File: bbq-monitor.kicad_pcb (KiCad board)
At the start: 4 copper layers, 48.5 x 43.3 mm, 51 parts, among them J1 Power, J2 USB_B_Mini, J3 Thermocouple, Q1 AO3401A, Q2 BC847, Q3 BC847, SW1 SW_Push, U1 ESP32-WROOM-32D, U2 TPS62132, U3 CP2104, U4 USBLC6-2SC6, U5 AD8495, U6 DHT11

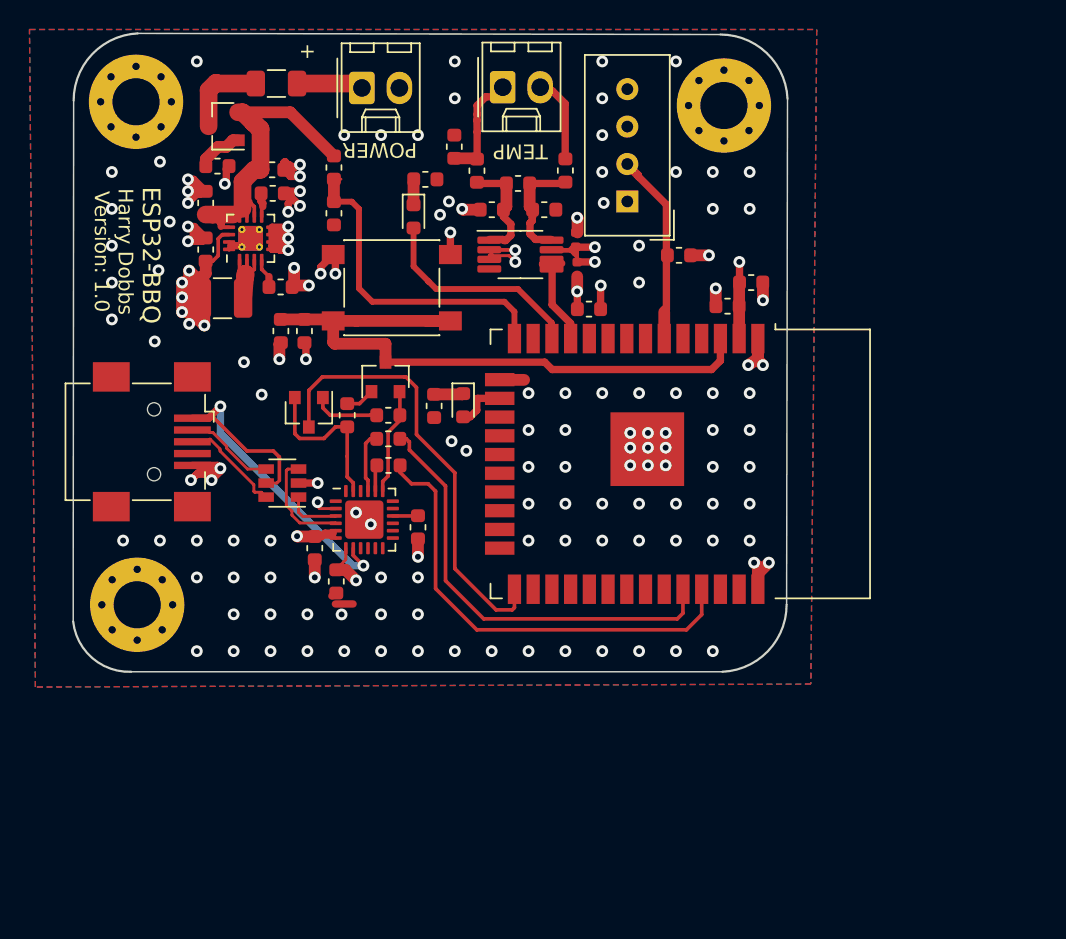
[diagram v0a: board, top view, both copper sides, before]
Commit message: up
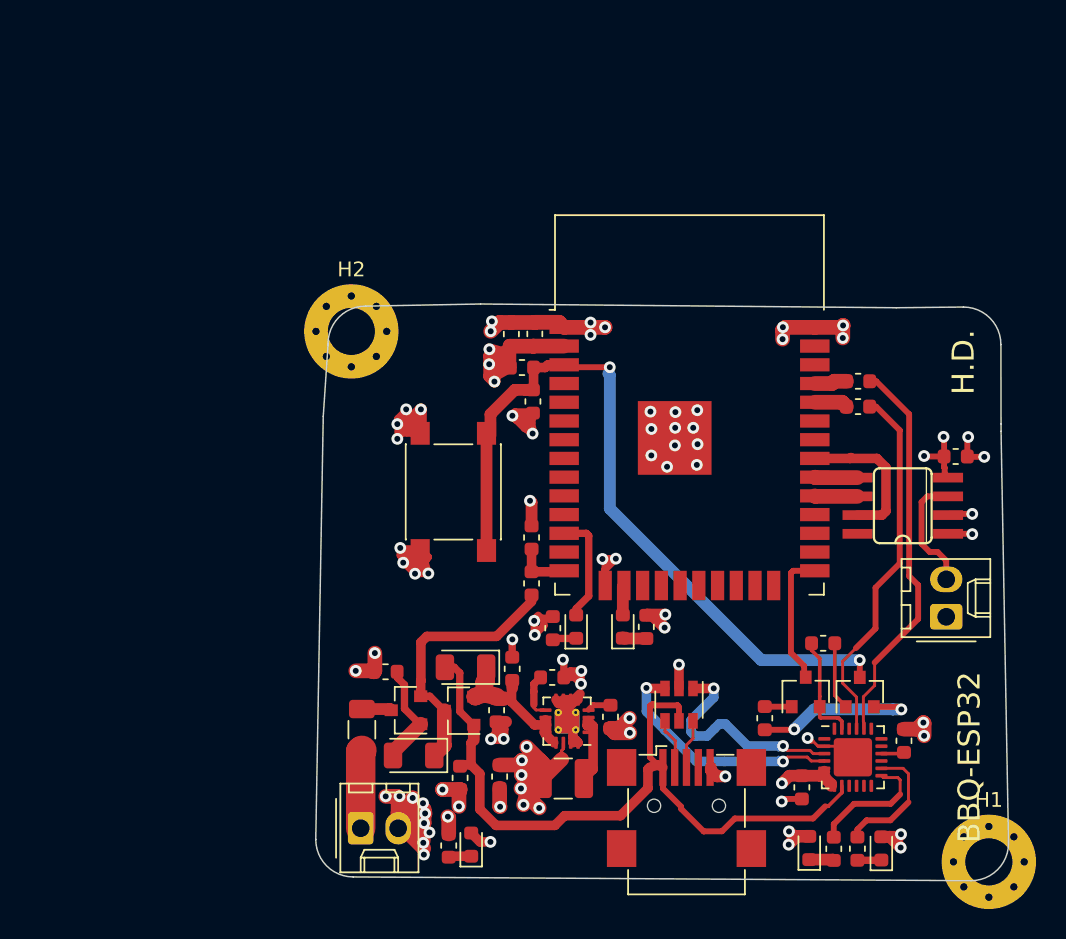
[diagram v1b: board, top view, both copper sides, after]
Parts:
- removed C10, C12, C14: 100n, Capacitor_SMD:C_0603_1608Metric
- removed C13, C15: 10n, Capacitor_SMD:C_0603_1608Metric
- removed C16: 100n, Capacitor_SMD:C_0402_1005Metric
- removed C17: 10u, Capacitor_SMD:C_0402_1005Metric
- removed H4: TR, MountingHole:MountingHole_3.2mm_M3_Pad_Via
- removed U5: AD8495, Package_SO:MSOP-8_3x3mm_P0.65mm
- removed U6: DHT11, Sensor:Aosong_DHT11_5.5x12.0_P2.54mm
- added C9: 100n, Capacitor_SMD:C_0603_1608Metric, F.Cu at (206.5, 86.8)
- added D3: RED, LED_SMD:LED_0603_1608Metric, F.Cu at (173.6, 113.1)
- added D4: RED, LED_SMD:LED_0603_1608Metric, F.Cu at (201.4, 113.4)
- added D5: RED, LED_SMD:LED_0603_1608Metric, F.Cu at (196.5, 113.4)
- added D6: D_Zener, Diode_SMD:D_1206_3216Metric, F.Cu at (169.7, 107.1)
- added D7: D_Schottky, Diode_SMD:D_1206_3216Metric, F.Cu at (173.2, 101.1)
- added IC1: MAX6675, hardware libraries:SO08, F.Cu at (202.9, 90.1)
- added Q4: AO3401A, Package_TO_SOT_SMD:SOT-23, F.Cu at (172.8, 104.0)
- J1: value Power -> Battery Power
- R10, R11, R9: value 1M -> 220
- R13: value 100 -> 10k
- moved H1 60.3 mm to (208.7, 114.3)
- moved R11 52.0 mm to (198.2, 113.4)
- moved J1 50.2 mm to (166.1, 112.0)
- moved R10 50.1 mm to (199.8, 113.4)
- moved R9 47.4 mm to (172.1, 113.2)
- moved J3 46.9 mm to (205.8, 97.7), turned to 90 degrees
- moved F1 44.2 mm to (166.2, 105.3), turned to 270 degrees
- moved J2 43.7 mm to (188.2, 110.5), turned to 0 degrees
- moved Q1 41.5 mm to (169.2, 104.0)
- moved C8 40.9 mm to (175.5, 108.5), turned to 270 degrees
- moved L1 39.9 mm to (179.9, 108.6)
- moved C1 39.7 mm to (175.3, 104.0), turned to 270 degrees
- moved U2 39.2 mm to (180.1, 104.8), turned to 180 degrees
- moved Q2 38.7 mm to (196.3, 102.8), turned to 90 degrees
- moved Q3 38.6 mm to (200.0, 102.8)
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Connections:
- net Net-(F1-Pad2) renamed BATT_PWR
- C1 pad 1: /BATT -> Net-(C1-Pad1)
- C2 pad 1: /BATT -> Net-(C1-Pad1)
- J2 pad 1: +5V -> USB_PWR
- J3 pad 1: Net-(J3-Pad1) -> GND
- J3 pad 2: Net-(J3-Pad2) -> Net-(IC1-Pad3)
- Q1 pad 2: /BATT -> BATT_SAFE
- R10 pad 1: Net-(J3-Pad2) -> TX_LED
- R10 pad 2: /Thermocouple_INPUT_FILTERED+ -> Net-(D4-Pad1)
- R11 pad 1: Net-(J3-Pad1) -> RX_LED
- R11 pad 2: /Thermocouple_INPUT_FILTERED- -> Net-(D5-Pad1)
- R12 pad 1: +3V3 -> GND
- R12 pad 2: TEMP_HUMID_SEN -> USB_PWR
- R14 pad 1: /BATT -> BATT_SAFE
- R9 pad 2: Net-(J3-Pad1) -> Net-(D3-Pad1)
- U1 pad 11: THERMOCOUPLE -> Net-(U1-Pad11)
- U1 pad 29: Net-(U1-Pad29) -> THERMO_SPI_CS
- U1 pad 30: Net-(U1-Pad30) -> THERMO_SPI_CLK
- U1 pad 31: Net-(U1-Pad31) -> THERMO_SPI_DO
- U1 pad 6: TEMP_HUMID_SEN -> Net-(U1-Pad6)
- U2 pad 10: /BATT -> Net-(C1-Pad1)
- U2 pad 11: /BATT -> Net-(C1-Pad1)
- U2 pad 12: /BATT -> Net-(C1-Pad1)
- U2 pad 13: /BATT -> Net-(C1-Pad1)
- U3 pad 13: Net-(U3-Pad13) -> RX_LED
- U3 pad 14: Net-(U3-Pad14) -> TX_LED
- U3 pad 8: +5V -> USB_PWR
- U4 pad 5: +5V -> USB_PWR
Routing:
- net USB_PWR: track 0.00 -> 51.1 mm
- net GND: track 71.2 -> 117.4 mm, vias 141 -> 68
- net /DIFF+: track 31.9 -> 2.22 mm
- net /DIFF-: track 30.7 -> 2.27 mm
- net +5V: track 27.4 -> 0.00 mm, vias 2 -> 0
- net /BATT: track 26.2 -> 0.00 mm
- net RX_CP+: track 1.78 -> 26.7 mm
- net GPIO0: track 30.3 -> 9.16 mm
- net TX_CP-: track 4.18 -> 24.9 mm
- net BATT_LEVEL: track 22.3 -> 3.78 mm
- net BATT_SAFE: track 0.00 -> 18.1 mm
- net TEMP_HUMID_SEN: track 14.3 -> 0.00 mm
- net Net-(C1-Pad1): track 0.00 -> 14.1 mm
- net D+: track 3.68 -> 15.7 mm, vias 0 -> 2
- net THERMO_SPI_DO: track 0.00 -> 10.2 mm
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- removed copper zone on B.Cu, net GND
- removed copper zone on F.Cu, net GND
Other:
- board size 48.5 x 43.3 mm -> 47 x 39.1 mm
- board text added: "BBQ-ESP32"
- board text added: "H.D."
- board text removed: "+"
- board text removed: "ESP32-BBQ"
- board text removed: "Harry Dobbs Version: 1.0"
- board text removed: "POWER"
- board text removed: "TEMP"
